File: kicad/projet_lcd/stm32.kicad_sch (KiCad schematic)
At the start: 24 parts, among them Y1 NI, Y2 32.768KHz

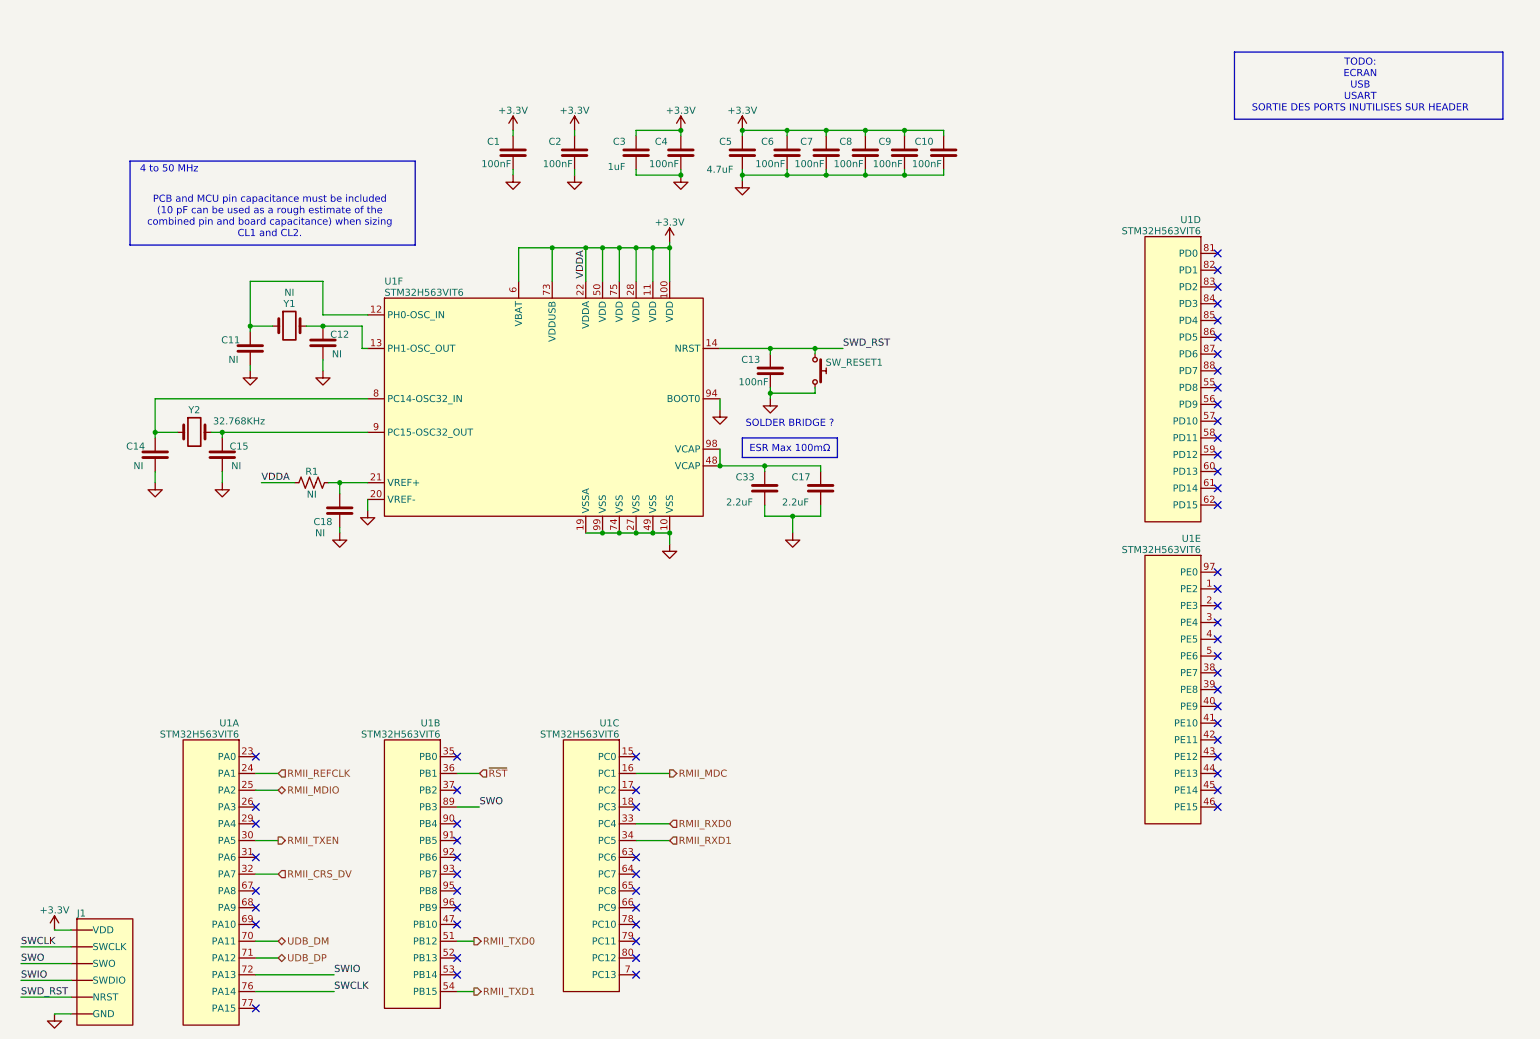
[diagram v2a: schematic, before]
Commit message: EOD
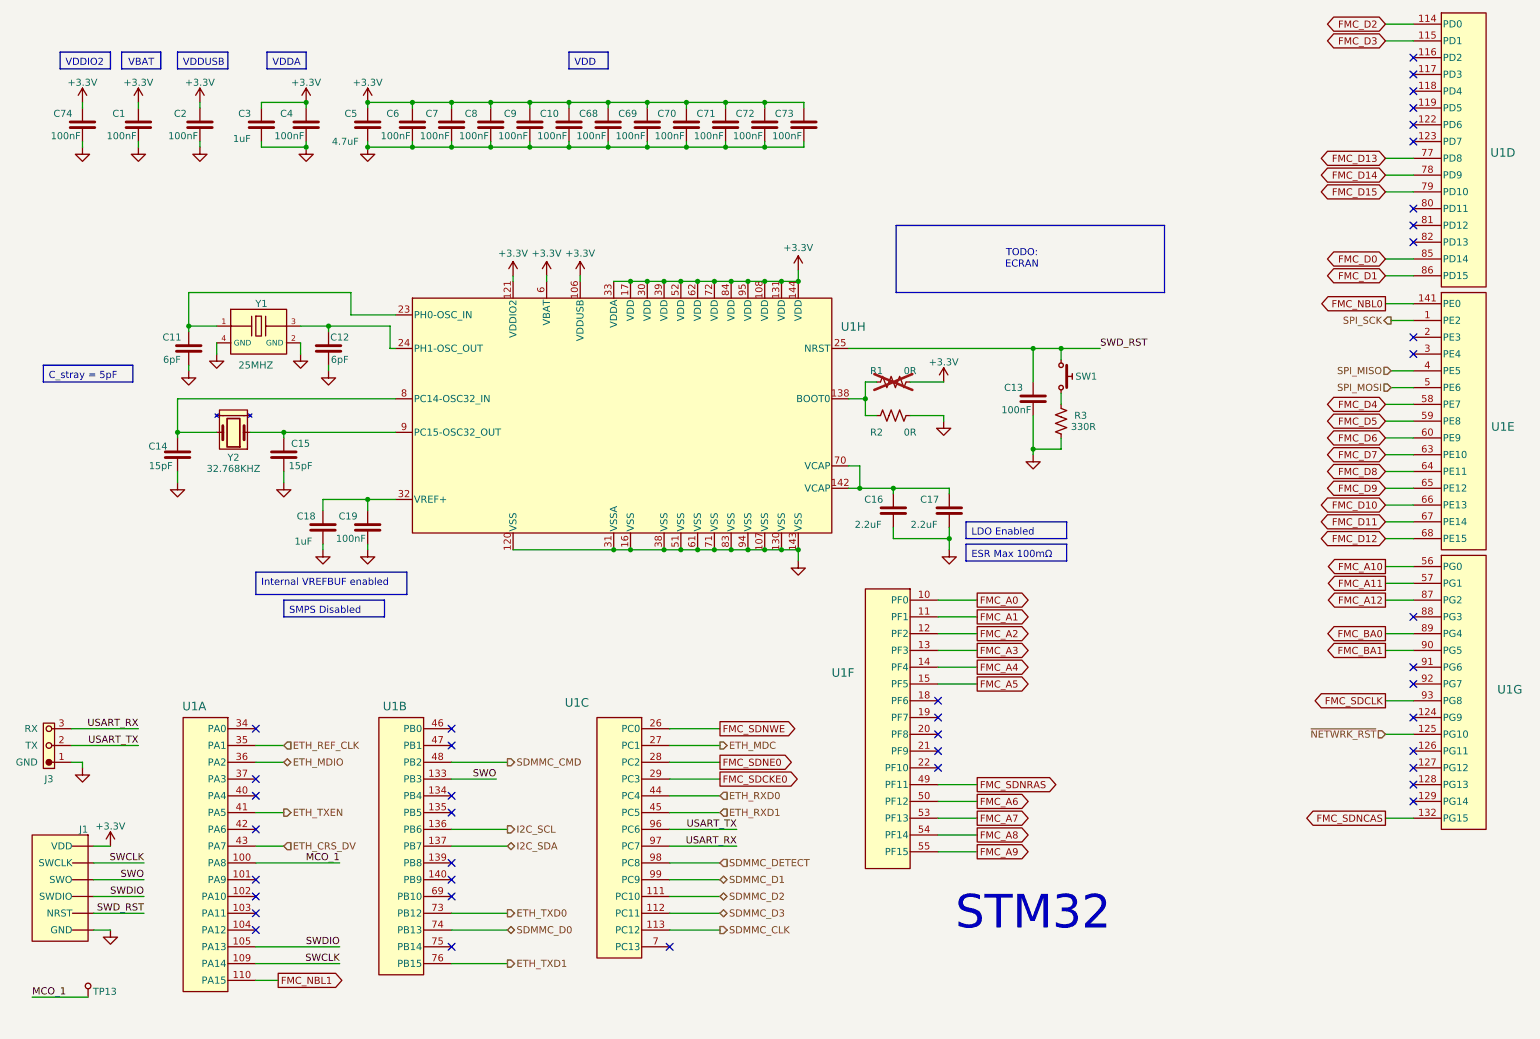
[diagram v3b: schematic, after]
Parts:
- removed U1: ~, Microcontrollers:STM32H563VIT6, symbol MicroControllers:STM32H563VIT6
- removed Y1: NI, symbol Generics:Y
- removed Y2: 32.768KHz, symbol Generics:Y
- added C19, C68, C69, C70, C71, C72, C73, C74: 100nF, Generics:C_0603, symbol Generics:C
- added J3: ~, Generics:Header_1x03_2.54_TH, symbol Generics:J_Connector_1x03
- added R2: 0R, Generics:R_0603, symbol Generics:R
- added R3: 330R, Generics:R_0603, symbol Generics:R
- added TP13: ~, PCB_Utils:TP_1.5, symbol PCB_Utils:TP
- added U1: STM32H563ZIT6, Microcontrollers:LQFP-144_STM-M, symbol MicroControllers:STM32H563ZIT6
- added Y1: 25MHZ, Crystals:NX2016SA-25MHZ-STD-CZS-2, symbol Crystals:NX2016SA-25MHZ-STD-CZS-2
- added Y2: 32.768KHZ, Crystals:ABS25-32.768KHZ-T, symbol Crystals:ABS25-32.768KHZ
- C11, C12: value NI -> 6pF; footprint (none) -> Generics:C_0402; LCSC Part # (none) -> C1575
- C14, C15: value NI -> 15pF; footprint (none) -> Generics:C_0402; LCSC Part # (none) -> C1548
- C18: value NI -> 1uF; footprint (none) -> Generics:C_0603; LCSC Part # (none) -> C15849
- R1: value NI -> 0R; footprint (none) -> Generics:R_0603; LCSC Part # (none) -> C21189; now not fitted; now left out of the parts list
- renumbered C33 to C16, SW_RESET1 to SW1
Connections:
- net +3.3V: now also R1.2 (1), C68.2, C69.2, C70.2, C71.2, C72.2, C73.2, C74.2, U1.106 (VDDUSB), U1.108 (VDD), U1.121 (VDDIO2), U1.131 (VDD), U1.144 (VDD), U1.17 (VDD), U1.30 (VDD), U1.33 (VDDA), U1.39 (VDD), U1.52 (VDD), U1.6 (VBAT), U1.62 (VDD), U1.72 (VDD), U1.84 (VDD), U1.95 (VDD); no longer R1.1
- net GND: now also C19.1, C68.1, C69.1, C70.1, C71.1, C72.1, C73.1, C74.1, J3.1, R2.2 (1), R3.1, U1.107 (VSS), U1.120 (VSS), U1.130 (VSS), U1.143 (VSS), U1.16 (VSS), U1.31 (VSSA), U1.38 (VSS), U1.51 (VSS), U1.61 (VSS), U1.71 (VSS), U1.83 (VSS), U1.94 (VSS), Y1.2 (GND), Y1.4 (GND); no longer SW1.2
- net SWCLK: now also U1.109 (PA14)
- net SWD_RST: now also U1.25 (NRST)
- net SWO: now also U1.133 (PB3)
- net at C16.2, C17.2: now also U1.142 (VCAP), U1.70 (VCAP)
- net at C15.2: now also U1.9 (PC15-OSC32_OUT), Y2.4
- net at C11.2: now also U1.23 (PH0-OSC_IN), Y1.1
- net at C12.2: now also U1.24 (PH1-OSC_OUT), Y1.3
- net at C18.2: now also C19.2, U1.32 (VREF+); no longer R1.2 (1)
- net at C14.2: now also U1.8 (PC14-OSC32_IN), Y2.1
- net SWIO renamed SWDIO
- net SWDIO: now also U1.105 (PA13)
- new net: R1.1, R2.1, U1.138 (BOOT0)
- new net: R3.2 (1), SW1.2
- new net ETH_CRS_DV: U1.43 (PA7)
- new net ETH_MDC: U1.27 (PC1)
- new net ETH_MDIO: U1.36 (PA2)
- new net ETH_REF_CLK: U1.35 (PA1)
- new net ETH_RXD0: U1.44 (PC4)
- new net ETH_RXD1: U1.45 (PC5)
- new net ETH_TXD0: U1.73 (PB12)
- new net ETH_TXD1: U1.76 (PB15)
- new net ETH_TXEN: U1.41 (PA5)
- new net FMC_A0: U1.10 (PF0)
- new net FMC_A1: U1.11 (PF1)
- new net FMC_A10: U1.56 (PG0)
- new net FMC_A11: U1.57 (PG1)
- new net FMC_A12: U1.87 (PG2)
- new net FMC_A2: U1.12 (PF2)
- new net FMC_A3: U1.13 (PF3)
- new net FMC_A4: U1.14 (PF4)
- new net FMC_A5: U1.15 (PF5)
- new net FMC_A6: U1.50 (PF12)
- new net FMC_A7: U1.53 (PF13)
- new net FMC_A8: U1.54 (PF14)
- new net FMC_A9: U1.55 (PF15)
- new net FMC_BA0: U1.89 (PG4)
- new net FMC_BA1: U1.90 (PG5)
- new net FMC_D0: U1.85 (PD14)
- new net FMC_D1: U1.86 (PD15)
- new net FMC_D10: U1.66 (PE13)
- new net FMC_D11: U1.67 (PE14)
- new net FMC_D12: U1.68 (PE15)
- new net FMC_D13: U1.77 (PD8)
- new net FMC_D14: U1.78 (PD9)
- new net FMC_D15: U1.79 (PD10)
- new net FMC_D2: U1.114 (PD0)
- new net FMC_D3: U1.115 (PD1)
- new net FMC_D4: U1.58 (PE7)
- new net FMC_D5: U1.59 (PE8)
- new net FMC_D6: U1.60 (PE9)
- new net FMC_D7: U1.63 (PE10)
- new net FMC_D8: U1.64 (PE11)
- new net FMC_D9: U1.65 (PE12)
- new net FMC_NBL0: U1.141 (PE0)
- new net FMC_NBL1: U1.110 (PA15)
- new net FMC_SDCKE0: U1.29 (PC3)
- new net FMC_SDCLK: U1.93 (PG8)
- new net FMC_SDNCAS: U1.132 (PG15)
- new net FMC_SDNE0: U1.28 (PC2)
- new net FMC_SDNRAS: U1.49 (PF11)
- new net FMC_SDNWE: U1.26 (PC0)
- new net I2C_SCL: U1.136 (PB6)
- new net I2C_SDA: U1.137 (PB7)
- new net MCO_1: TP13.1, U1.100 (PA8)
- new net SDMMC_CLK: U1.113 (PC12)
- new net SDMMC_CMD: U1.48 (PB2)
- new net SDMMC_D0: U1.74 (PB13)
- new net SDMMC_D1: U1.99 (PC9)
- new net SDMMC_D2: U1.111 (PC10)
- new net SDMMC_D3: U1.112 (PC11)
- new net SDMMC_DETECT: U1.98 (PC8)
- new net SPI_MISO: U1.4 (PE5)
- new net SPI_MOSI: U1.5 (PE6)
- new net SPI_SCK: U1.1 (PE2)
- new net USART_RX: J3.3, U1.97 (PC7)
- new net USART_TX: J3.2, U1.96 (PC6)
- new net ~{NETWRK_RST}: U1.125 (PG10)
- no-connect marks 61 -> 41
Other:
- note added: "STM32"
- note added: "TODO: ECRAN"
- note removed: "4 to 50 MHz"
- note removed: "ESR Max 100mΩ"
- note removed: "PCB and MCU pin capacitance must be included (10 pF can be used as a rough estimate of the combined pin and board capacitance) when sizing CL1 and CL2."
- note removed: "SOLDER BRIDGE ?"
- note removed: "TODO: ECRAN USB USART SORTIE DES PORTS INUTILISES SUR HEADER"
- moved on the sheet: C1, C10, C11, C13, C14, C16, C17, C2, C3, C4, C5, C6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
